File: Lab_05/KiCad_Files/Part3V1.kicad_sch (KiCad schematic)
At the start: 26 parts, among them Q301 NPN, Q302 PNP, Q303 NPN, Q304 NPN, Q305 PNP

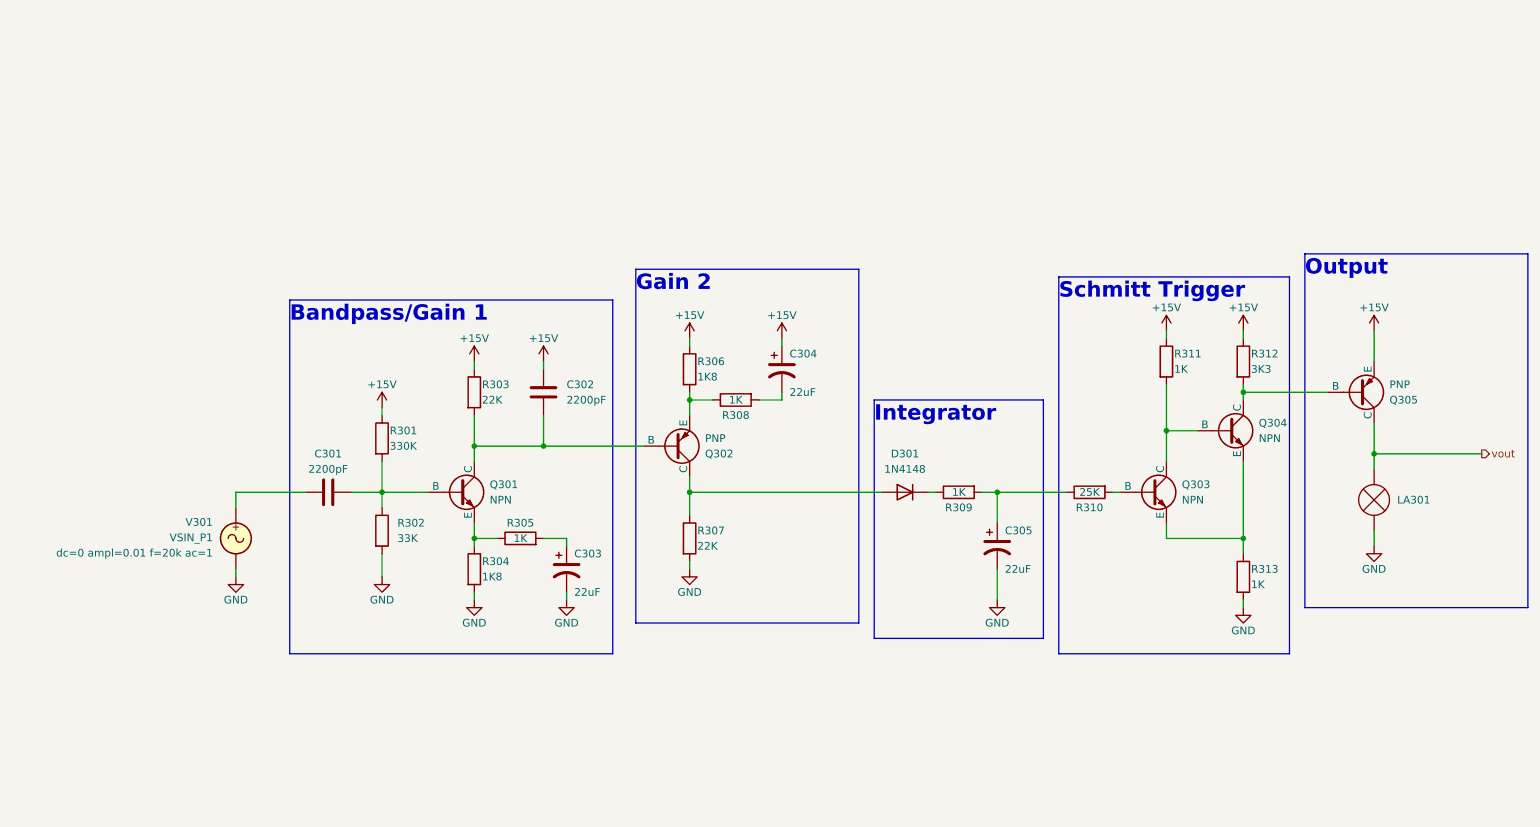
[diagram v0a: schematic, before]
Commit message: Finish Lab 5
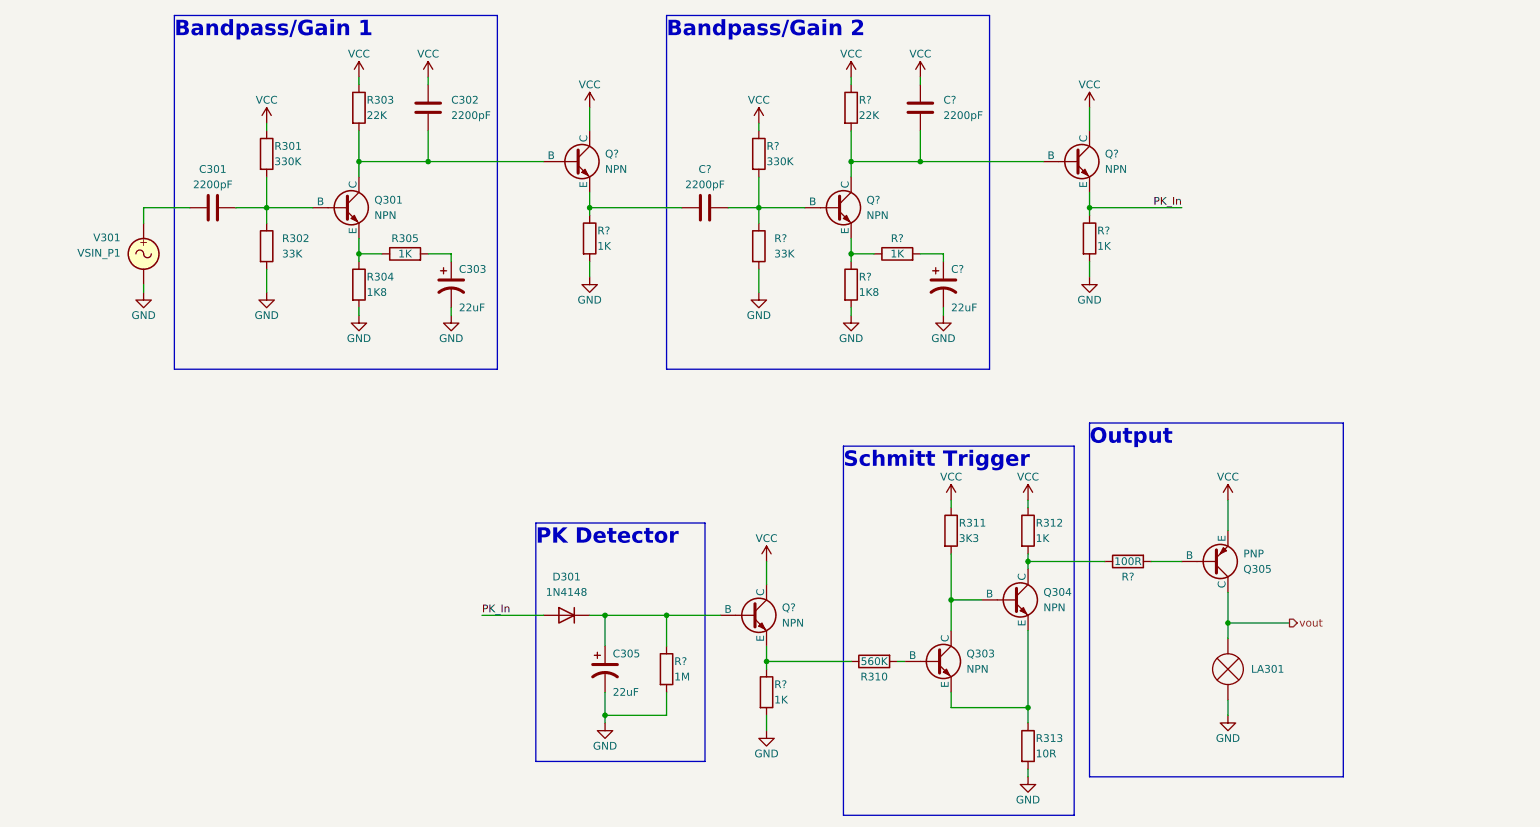
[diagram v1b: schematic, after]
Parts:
- removed C304: 22uF, symbol Device:C_Polarized_US
- removed Q302: PNP, symbol Simulation_SPICE:PNP
- removed R306: 1K8, symbol Device:R
- removed R307: 22K, symbol Device:R
- removed R308, R309: 1K, symbol Device:R
- added C?: 22uF, symbol Device:C_Polarized_US
- added C? (x2): 2200pF, symbol Device:C
- added Q? (x4): NPN, symbol Simulation_SPICE:NPN
- added R?: 1K8, symbol Device:R
- added R? (x4): 1K, symbol Device:R
- added R?: 22K, symbol Device:R
- added R?: 33K, symbol Device:R
- added R?: 1M, symbol Device:R
- added R?: 100R, symbol Device:R
- added R?: 330K, symbol Device:R
- R310: value 25K -> 560K
- R311: value 1K -> 3K3
- R312: value 3K3 -> 1K
- R313: value 1K -> 10R
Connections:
- net GND: now also C?.2, R?.2, R?.2, R?.2, R?.2, R?.2, R?.2
- net at D301.1 (K): now also C305.1, Q?.2 (B), R?.1
- net at R310.1: now also Q?.3 (E), R?.1; no longer C305.1
- net at C302.2, Q301.1 (C), R303.2: now also Q?.2 (B)
- net at Q304.1 (C), R312.2: now also R?.1; no longer Q305.2 (B)
- net PK_In: now reaches D301.2 (A)
- net PK_In: now also Q?.3 (E), R?.1
- net +15V renamed VCC
- net VCC: now also C?.1, Q?.1 (C), Q?.1 (C), Q?.1 (C), R?.1, R?.1
- new net: C?.1, R?.2
- new net: C?.1, Q?.3 (E), R?.1
- new net: C?.2, Q?.2 (B), R?.1, R?.2
- new net: Q?.3 (E), R?.1, R?.1
- new net: C?.2, Q?.1 (C), Q?.2 (B), R?.2
- new net: Q305.2 (B), R?.2
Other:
- note added: "Bandpass/Gain 2"
- note added: "PK Detector"
- note removed: "Gain 2"
- note removed: "Integrator"
- moved on the sheet: C301, C302, C303, C305, D301, LA301, Q301, Q303, Q304, Q305, R301, R302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
